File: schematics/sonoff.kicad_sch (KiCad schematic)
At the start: 18 parts, among them J1 Screw_Terminal_01x06, J2 Screw_Terminal_01x04, J3 Conn_02x03_Odd_Even, K1 Relay_SPDT, K2 Relay_SPDT, Q1 2N7000, Q2 2N7000, U1 ESP-01v090

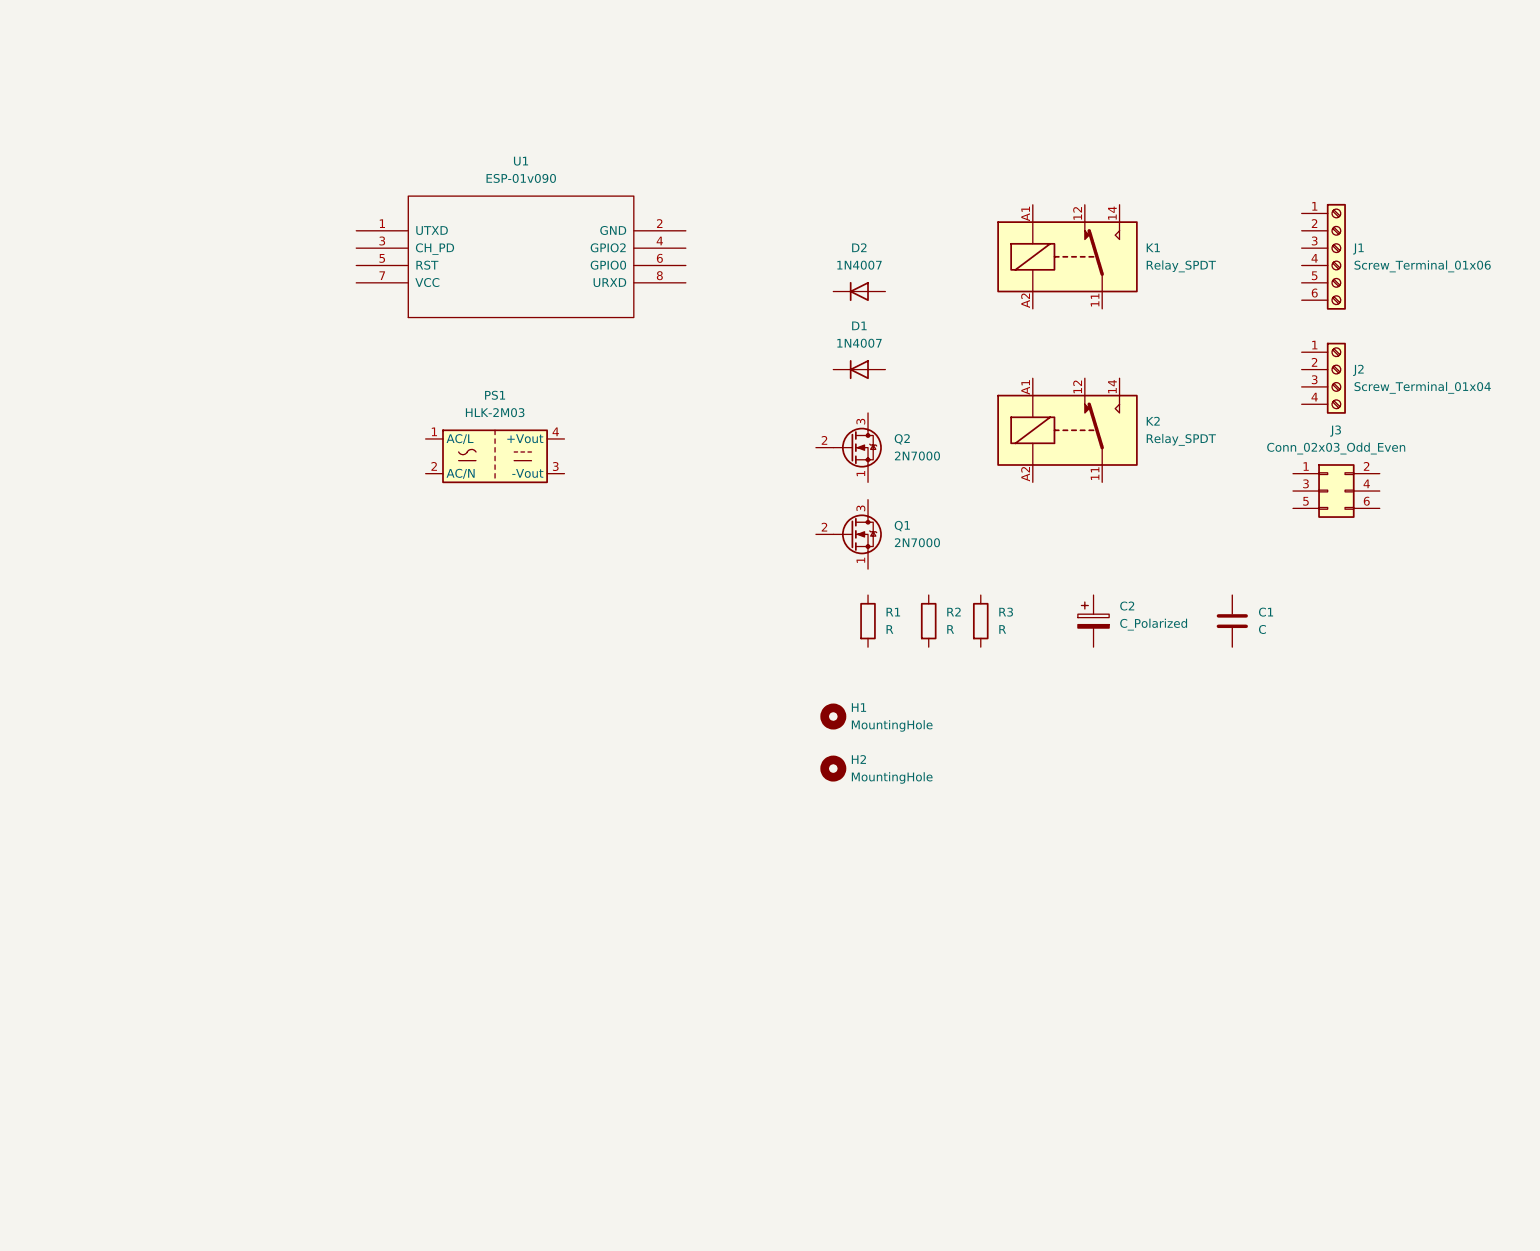
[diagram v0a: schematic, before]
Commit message: feat
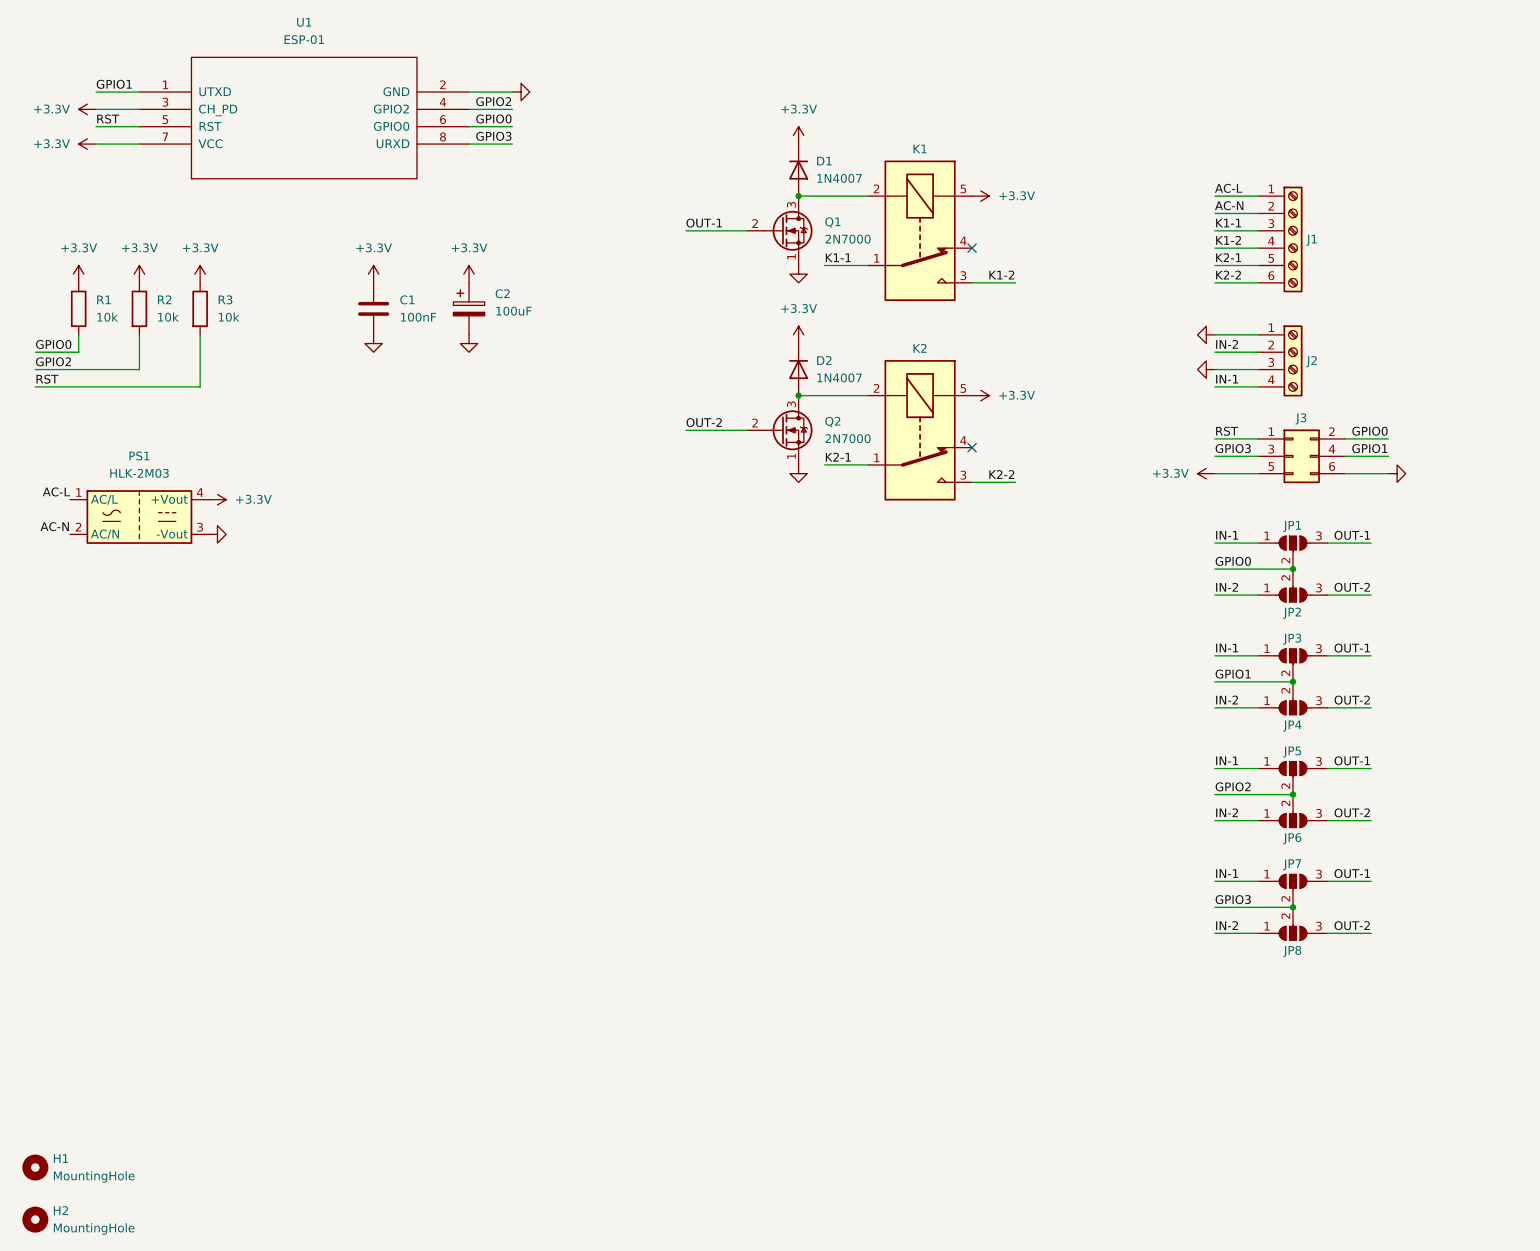
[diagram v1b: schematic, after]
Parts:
- added JP1, JP2, JP3, JP4, JP5, JP6, JP7, JP8: SolderJumper_3_Open, Jumper:SolderJumper-3_P1.3mm_Open_Pad1.0x1.5mm, symbol Jumper:SolderJumper_3_Open
- C1: value C -> 100nF
- C2: value C_Polarized -> 100uF
- R1, R2, R3: value R -> 10k
- U1: value ESP-01v090 -> ESP-01
- renumbered D2 to D1, D1 to D2, K2 to K1, K1 to K2
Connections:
- net GPIO1: now reaches U1.1 (UTXD)
- net GPIO1: now also J3.4 (Pin_4), JP3.2 (C), JP4.2 (C)
- net GND: now reaches U1.2 (GND)
- net GND: now also C1.2, C2.2, J2.1 (Pin_1), J2.3 (Pin_3), J3.6 (Pin_6), PS1.3 (-Vout), Q1.1 (S), Q2.1 (S)
- net +3.3V: now reaches U1.3 (CH_PD)
- net +3.3V: now also C1.1, C2.1, D1.1 (K), D2.1 (K), J3.5 (Pin_5), K1.5, K2.5, PS1.4 (+Vout), R1.1, R2.1, R3.1, U1.7 (VCC)
- net GPIO2: now reaches U1.4 (GPIO2)
- net GPIO2: now also R2.2, JP5.2 (C), JP6.2 (C)
- net RST: now reaches U1.5 (RST)
- net RST: now also J3.1 (Pin_1), R3.2
- net GPIO0: now reaches U1.6 (GPIO0)
- net GPIO0: now also J3.2 (Pin_2), R1.2, JP1.2 (C), JP2.2 (C)
- net GPIO3: now reaches U1.8 (URXD)
- net GPIO3: now also J3.3 (Pin_3), JP7.2 (C), JP8.2 (C)
- net OUT-2: now reaches Q2.2 (G)
- net OUT-2: now also JP2.3 (B), JP4.3 (B), JP6.3 (B), JP8.3 (B)
- net at Q2.3 (D): now also D2.2 (A), K2.2
- net AC-L: now reaches PS1.1 (AC/L)
- net AC-L: now also J1.1 (Pin_1)
- net AC-N: now reaches PS1.2 (AC/N)
- net AC-N: now also J1.2 (Pin_2)
- net at D1.2 (A): now also K1.2, Q1.3 (D)
- net OUT-1: now reaches Q1.2 (G)
- net OUT-1: now also JP1.3 (B), JP3.3 (B), JP5.3 (B), JP7.3 (B)
- net IN-2: now reaches J2.2 (Pin_2)
- net IN-2: now also JP2.1 (A), JP4.1 (A), JP6.1 (A), JP8.1 (A)
- net IN-1: now reaches J2.4 (Pin_4)
- net IN-1: now also JP1.1 (A), JP3.1 (A), JP5.1 (A), JP7.1 (A)
- net K1-1: now reaches J1.3 (Pin_3)
- net K1-1: now also K1.1
- net K1-2: now reaches J1.4 (Pin_4)
- net K1-2: now also K1.3
- net K2-1: now reaches J1.5 (Pin_5)
- net K2-1: now also K2.1
- net K2-2: now reaches J1.6 (Pin_6)
- net K2-2: now also K2.3
- no-connect marks 0 -> 2
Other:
- company: (none) -> Davide Scalisi
- title: (none) -> Sonoff
- moved on the sheet: C1, C2, D1, D2, H1, H2, J1, J2, J3, K1, K2, PS1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

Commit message: !feat: first rev2 release
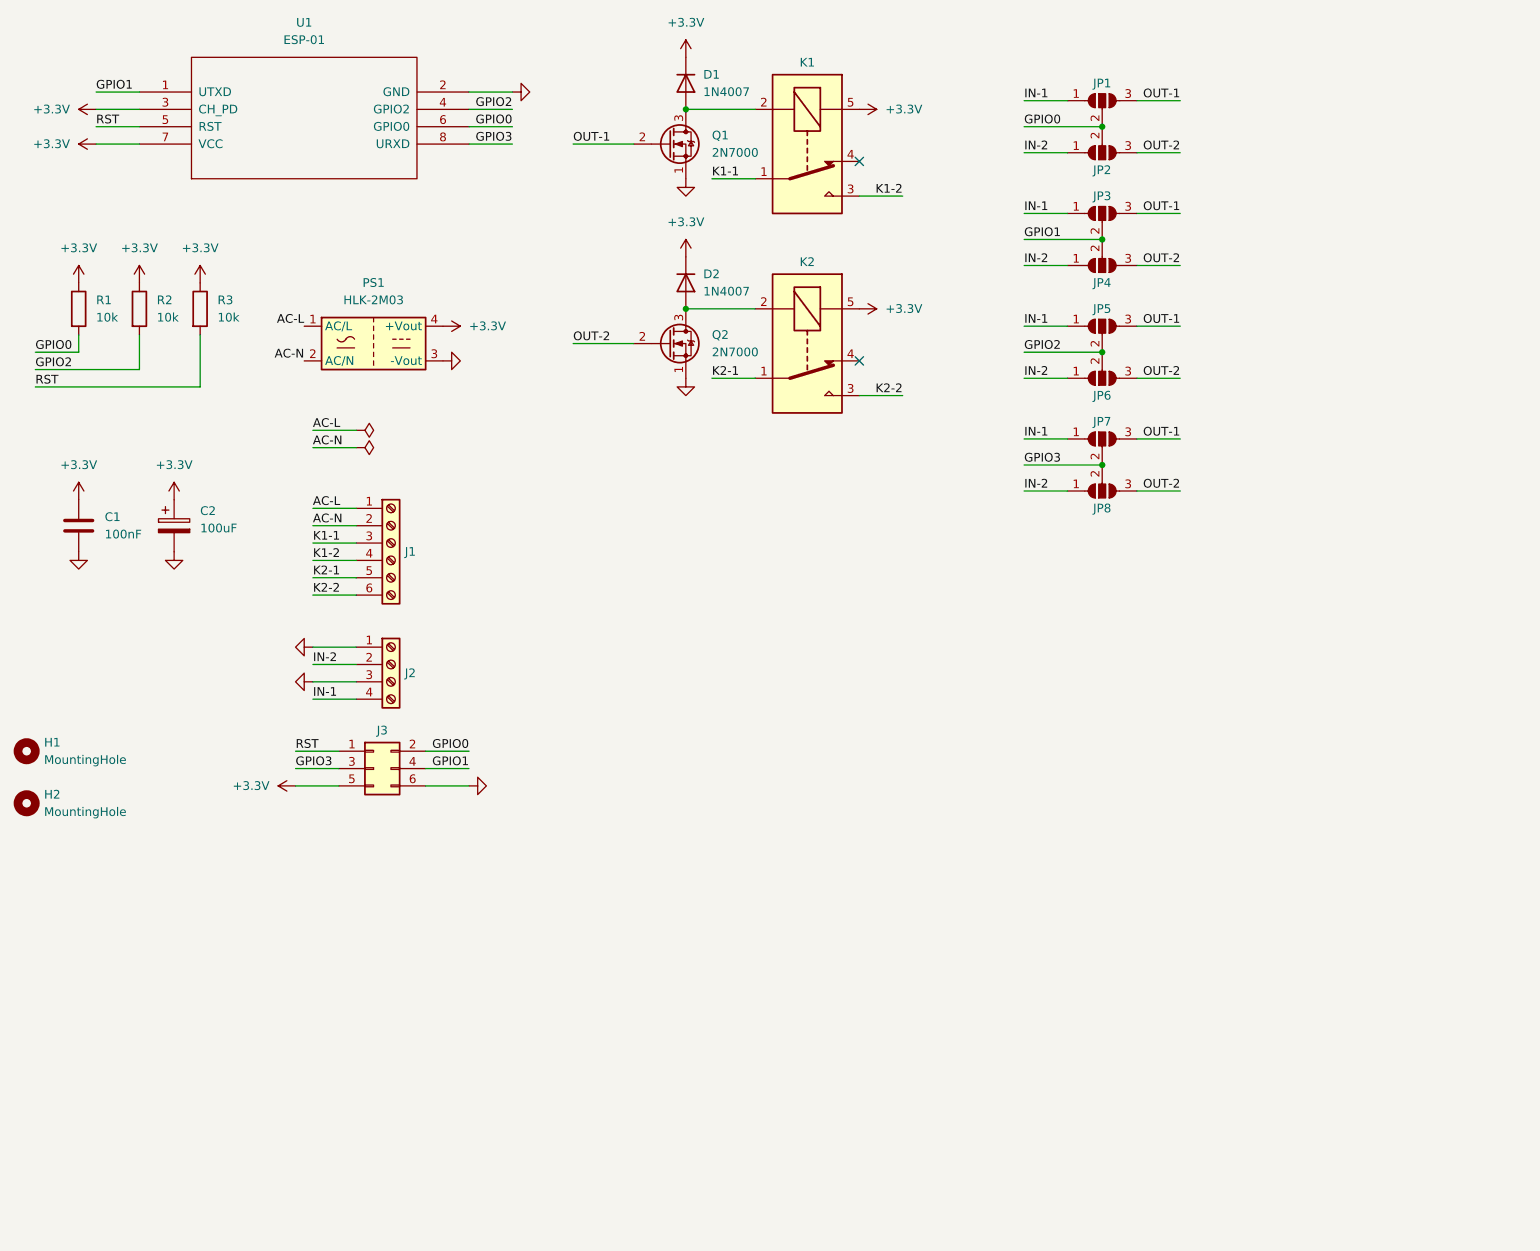
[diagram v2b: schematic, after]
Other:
- moved on the sheet: C1, C2, D1, D2, H1, H2, J1, J2, J3, JP1, JP2, JP3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
